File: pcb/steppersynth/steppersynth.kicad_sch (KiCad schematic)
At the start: 20 parts, among them J1 USB4105, J2 LRS-350-24, SW1 SW_SPST, U1 ESP32-S3-WROOM-2, U2 LM3940IMPX-3.3/NOPB

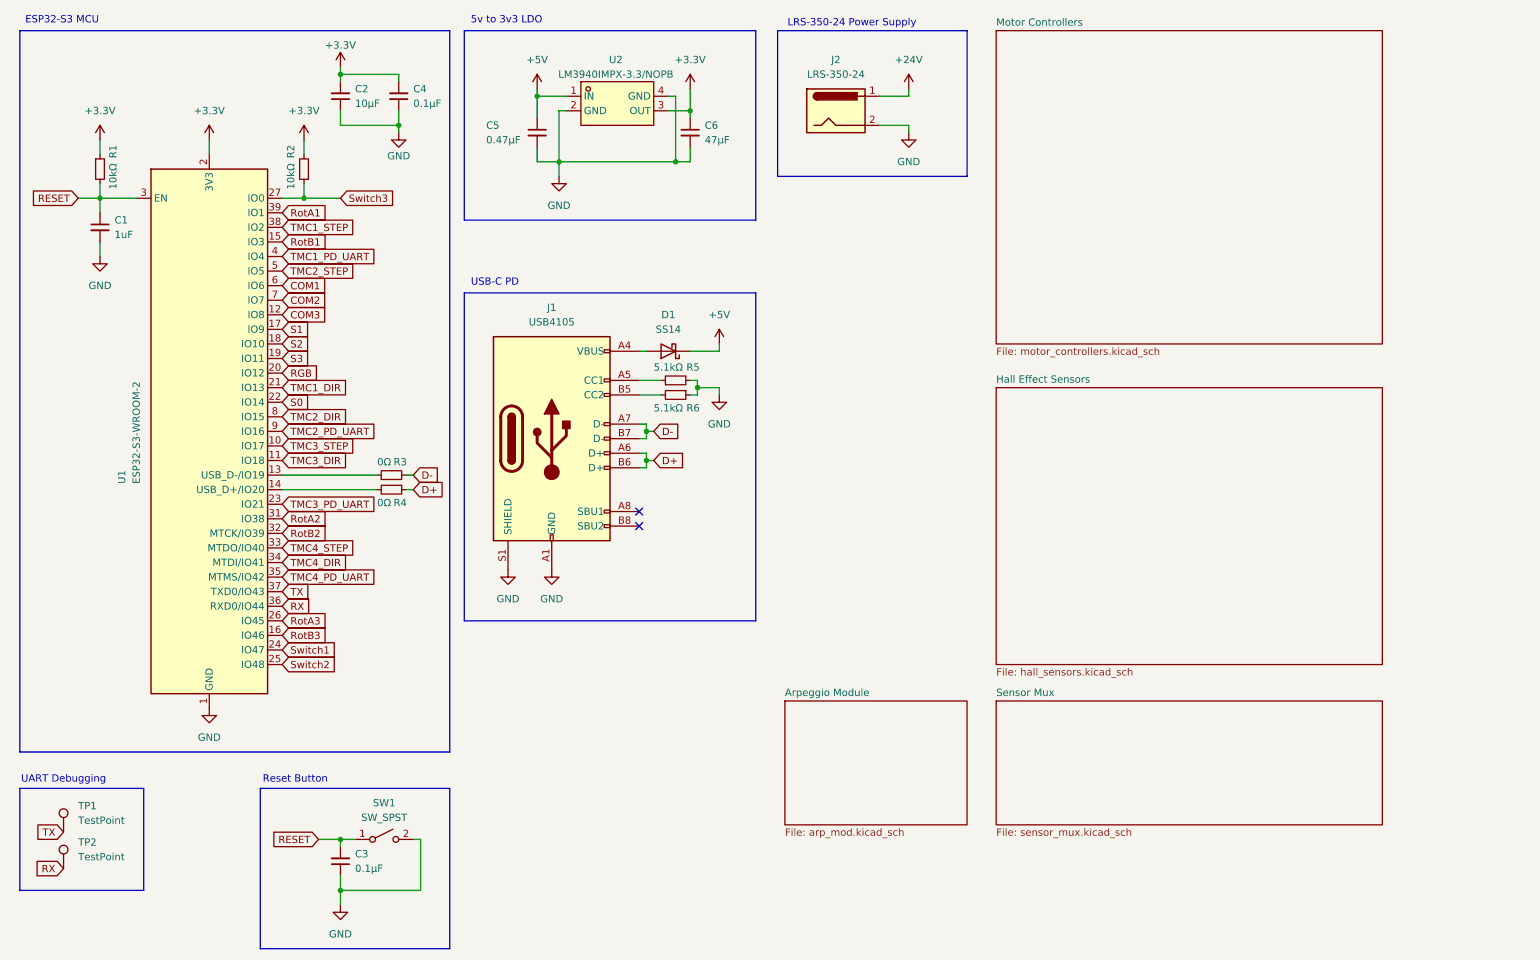
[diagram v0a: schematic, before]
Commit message: dc-dc buck converter
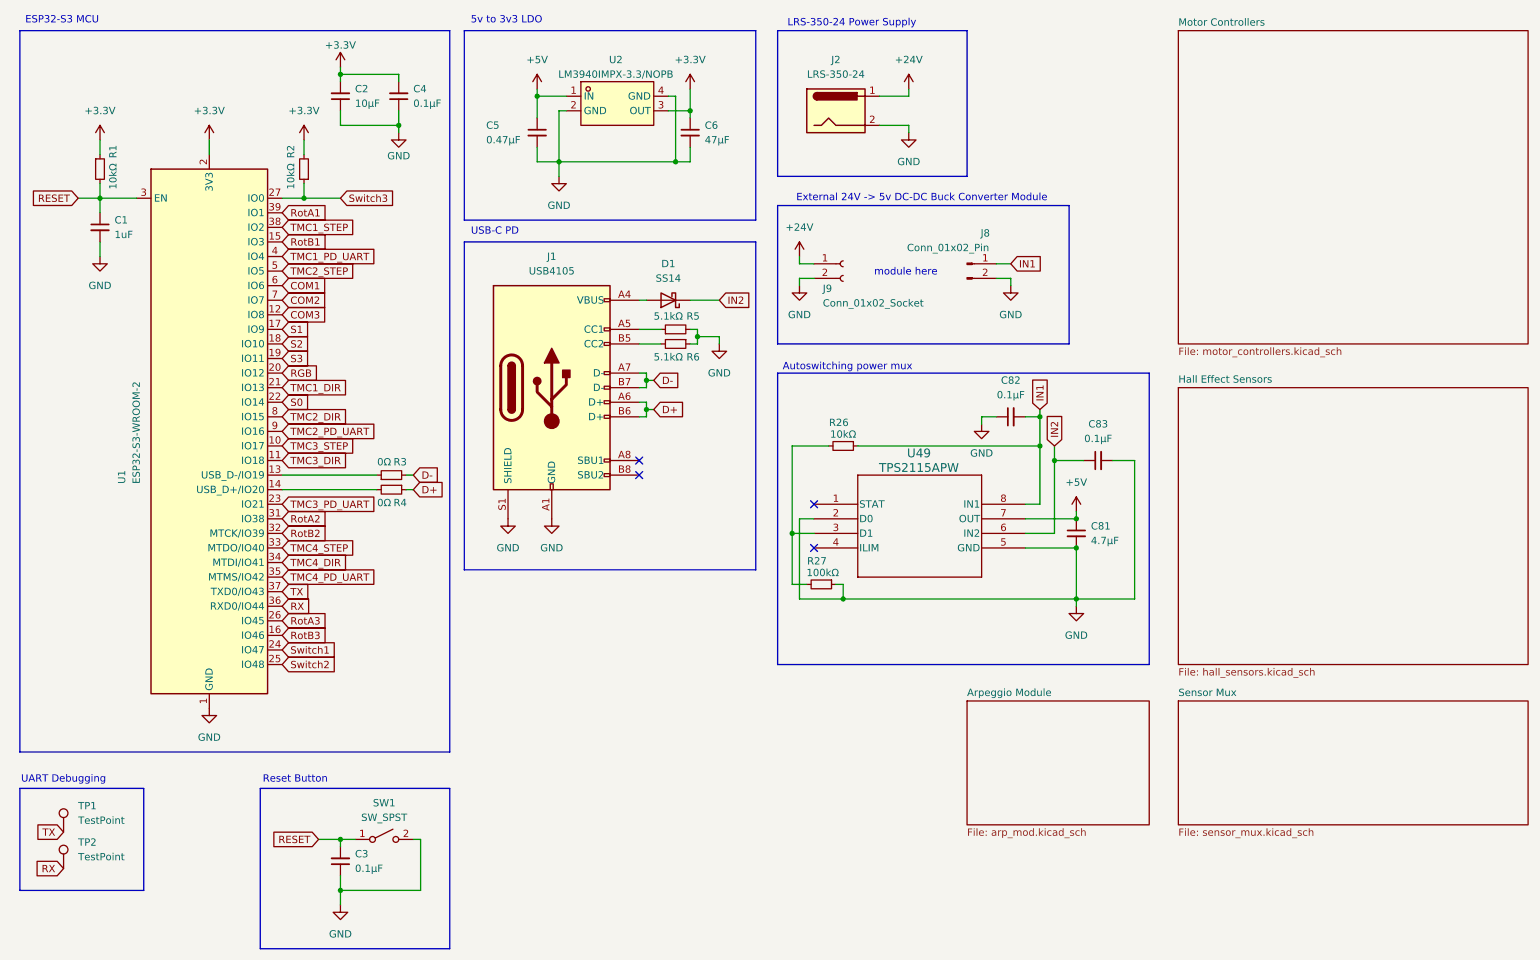
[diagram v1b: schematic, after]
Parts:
- added C81: 4.7μF, Capacitor_SMD:C_0805_2012Metric, symbol Device:C_Small
- added C82, C83: 0.1μF, Capacitor_SMD:C_0805_2012Metric, symbol Device:C_Small
- added J8: Conn_01x02_Pin, Connector_PinSocket_2.54mm:PinSocket_1x02_P2.54mm_Vertical, symbol Connector:Conn_01x02_Pin
- added J9: Conn_01x02_Socket, Connector_PinSocket_2.54mm:PinSocket_1x02_P2.54mm_Vertical, symbol Connector:Conn_01x02_Socket
- added R26: 10kΩ, Resistor_SMD:R_0805_2012Metric, symbol Device:R_Small
- added R27: 100kΩ, Resistor_SMD:R_0805_2012Metric, symbol Device:R_Small
- added U49: TPS2115APW, 2_udu_lib:PW8, symbol 3_udu_lib:TPS2115APW
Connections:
- net +24V: now also J9.1 (Pin_1)
- net +5V: now also C81.1, U49.7 (OUT); no longer D1.1 (K)
- net GND: now also C81.2, C82.1, C83.2, J8.2 (Pin_2), J9.2 (Pin_2), R27.1, U49.2 (D0), U49.5 (GND)
- new net: R26.2, R27.2, U49.3 (D1)
- new net IN1: C82.2, J8.1 (Pin_1), R26.1, U49.8 (IN1)
- new net IN2: C83.1, D1.1 (K), U49.6 (IN2)
- no-connect marks 2 -> 4
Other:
- note added: "Autoswitching power mux"
- note added: "External 24V -> 5v DC-DC Buck Converter Module"
- note added: "module here"
- moved on the sheet: D1, J1, R5, R6
